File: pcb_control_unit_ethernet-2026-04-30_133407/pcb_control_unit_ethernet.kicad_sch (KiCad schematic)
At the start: 42 parts, among them J1 STDC14, J2 Micro_SD_Card_Det1, SW1 Reset, SW2 Boot, U1 STM32H563VITx, U10 SIT3051TK

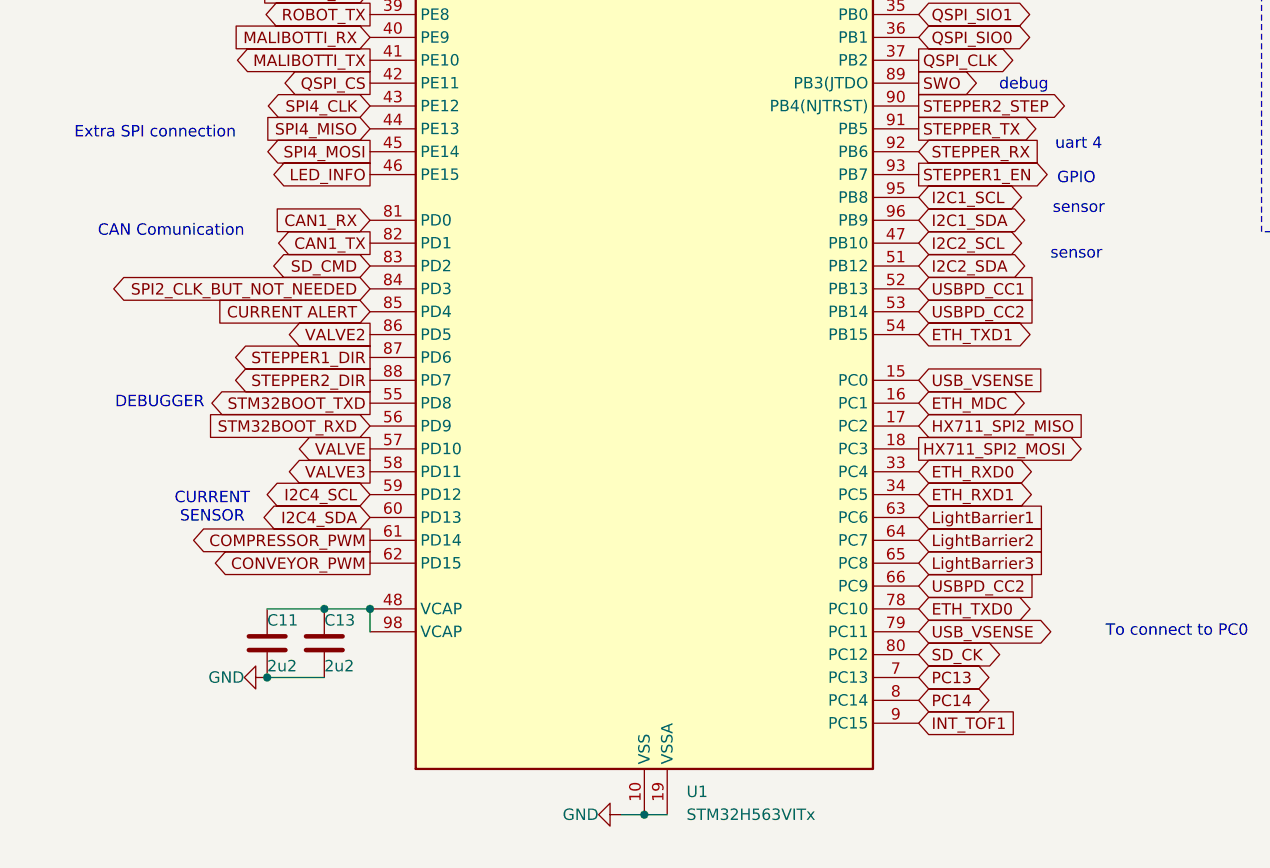
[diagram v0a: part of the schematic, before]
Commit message: WIP
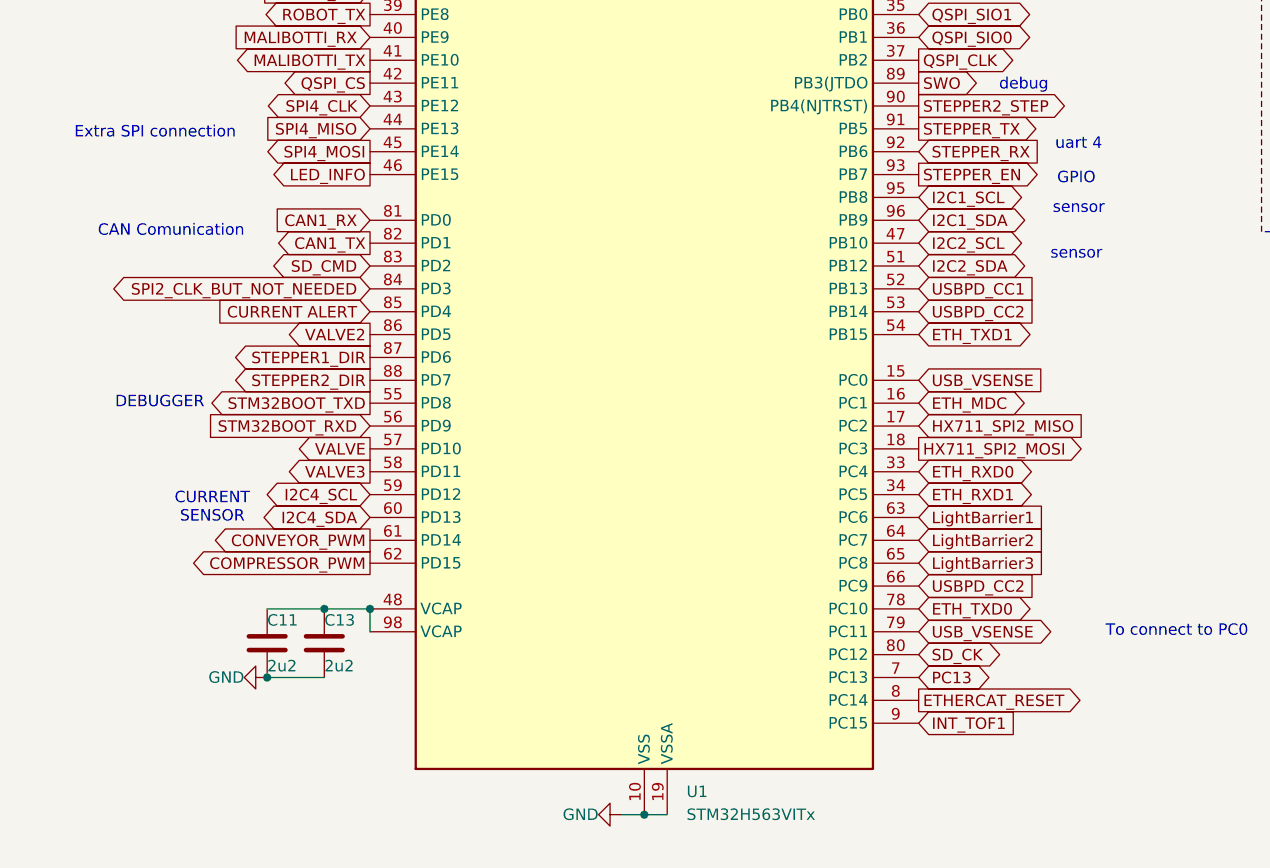
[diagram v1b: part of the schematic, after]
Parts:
- R1, R11, R12, R13, R14, R2, R3, R4, R5, R6, R63, R7, R8, R9: footprint Resistor_SMD:R_0201_0603Metric -> Resistor_SMD:R_0402_1005Metric
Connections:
- net COMPRESSOR_PWM: now also U1.62 (PD15); no longer U1.61 (PD14)
- net CONVEYOR_PWM: now also U1.61 (PD14); no longer U1.62 (PD15)
- net PC14 renamed ETHERCAT_RESET
- net STEPPER1_EN renamed STEPPER_EN

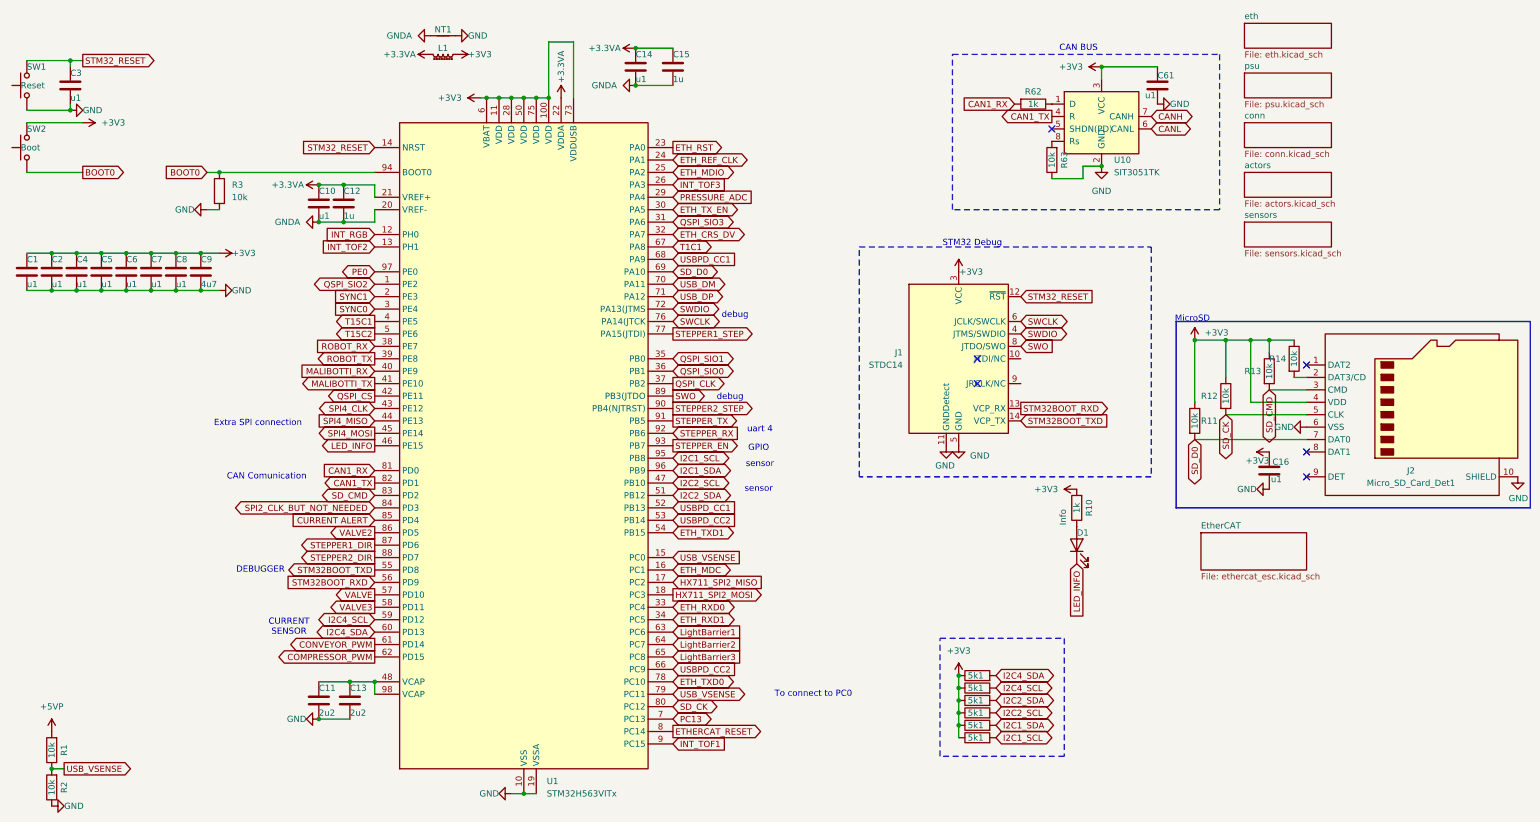
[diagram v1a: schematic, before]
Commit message: WIP
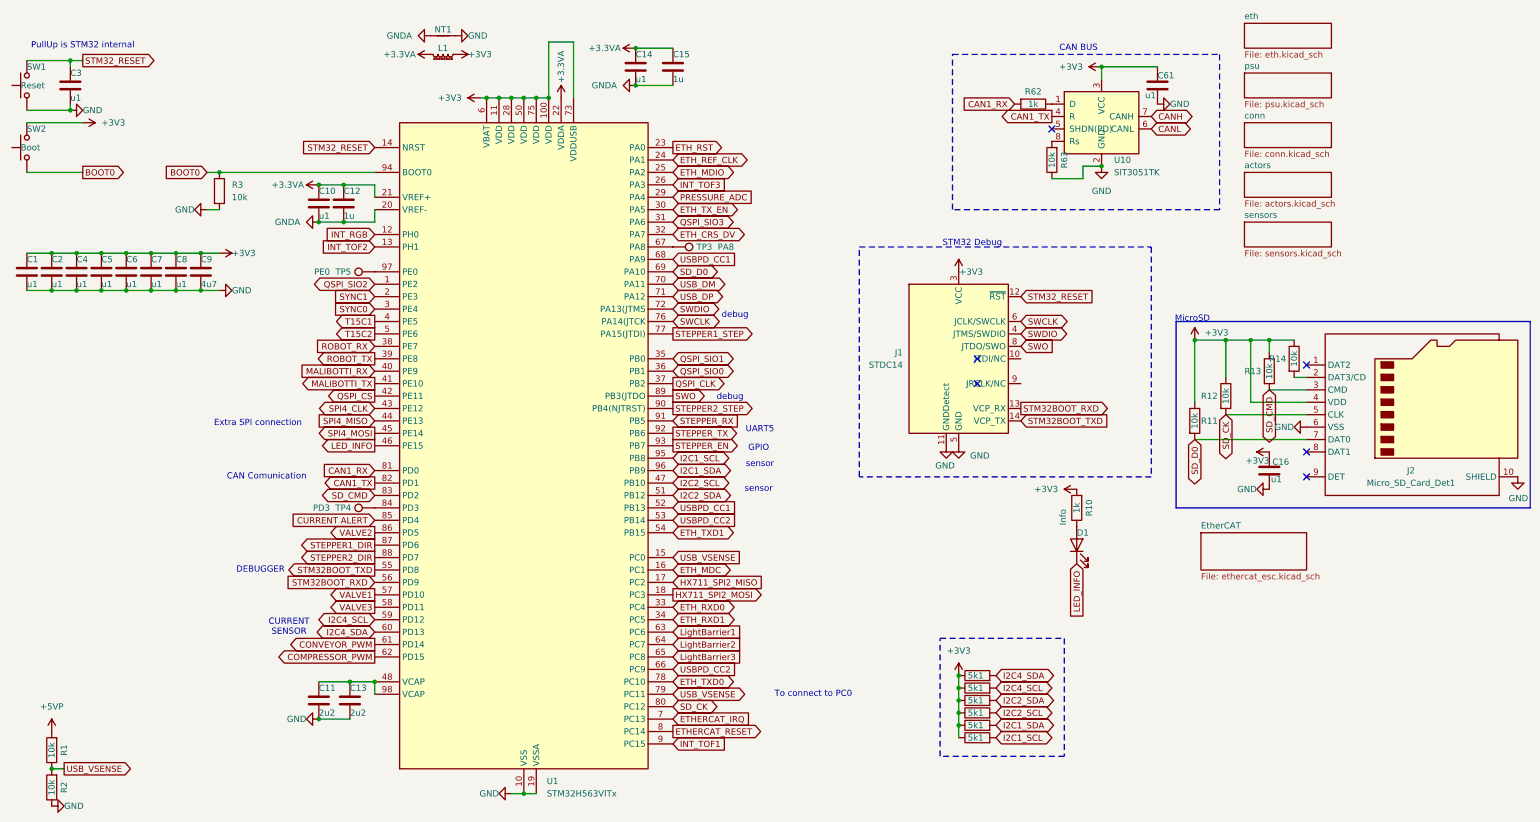
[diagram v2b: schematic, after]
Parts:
- added TP3: PA8, TestPoint:TestPoint_THTPad_D1.0mm_Drill0.5mm, symbol Connector:TestPoint
- added TP4: PD3, TestPoint:TestPoint_THTPad_D1.0mm_Drill0.5mm, symbol Connector:TestPoint
- added TP5: PE0, TestPoint:TestPoint_THTPad_D1.0mm_Drill0.5mm, symbol Connector:TestPoint
- L1: value 600R@100M -> 220R@100M
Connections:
- net STEPPER_RX: now also U1.91 (PB5); no longer U1.92 (PB6)
- net STEPPER_TX: now also U1.92 (PB6); no longer U1.91 (PB5)
- net PC13 renamed ETHERCAT_IRQ
- net PE0: no longer names the net of U1.97 (PE0)
- net PE0: now also TP5.1
- net SPI2_CLK_BUT_NOT_NEEDED: no longer names the net of U1.84 (PD3)
- net SPI2_CLK_BUT_NOT_NEEDED: now also TP4.1
- net T1C1: no longer names the net of U1.67 (PA8)
- net T1C1: now also TP3.1
- net VALVE renamed VALVE1
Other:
- note added: "PullUp is STM32 internal"
- note added: "UART5"
- note removed: "uart 4"
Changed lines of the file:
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@@
 (kicad_sch
-	(version 20250114)
+	(version 20260306)
 	(generator "eeschema")
-	(generator_version "9.0")
+	(generator_version "10.0")
 	(paper "A4")

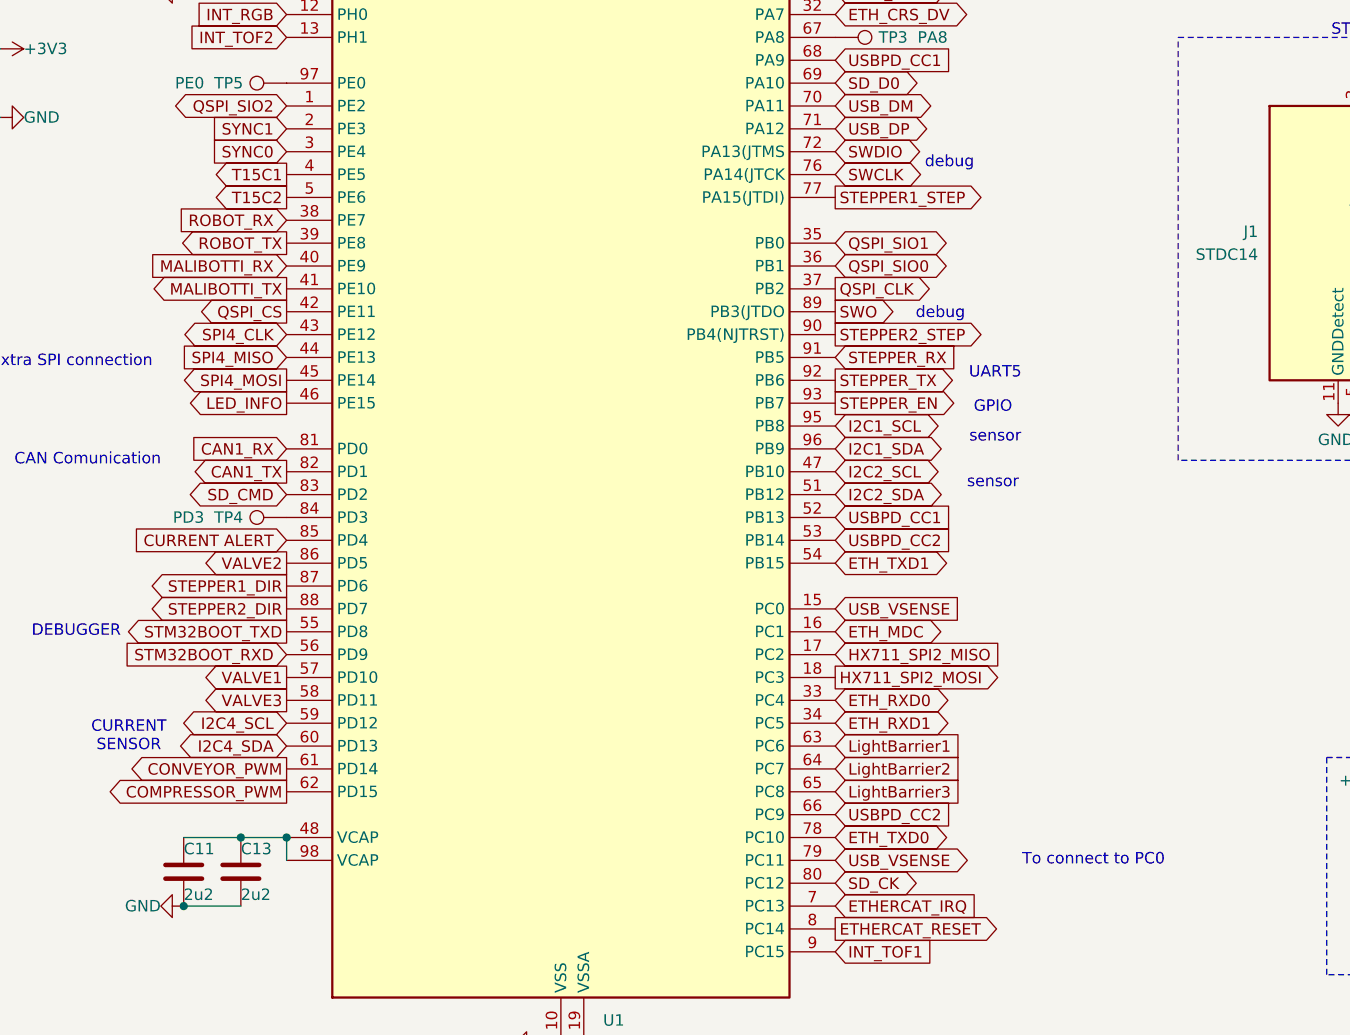
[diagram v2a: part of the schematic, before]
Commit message: Release Candidate
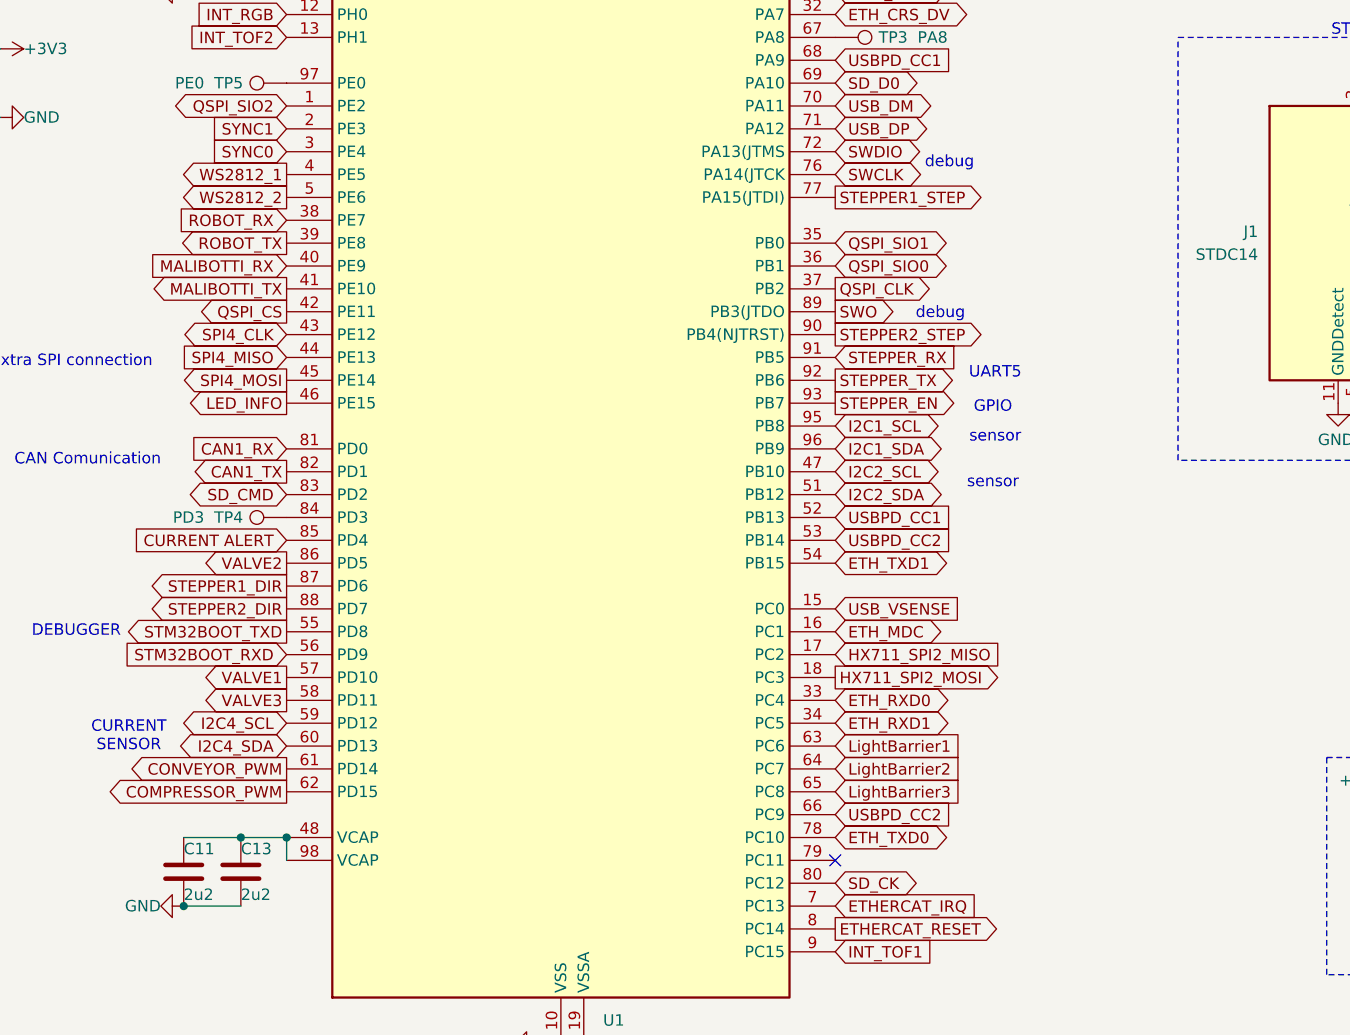
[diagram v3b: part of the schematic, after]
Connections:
- net USB_VSENSE: no longer U1.79 (PC11)
- net T15C1 renamed WS2812_1
- net T15C2 renamed WS2812_2
- no-connect marks 6 -> 7
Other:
- note removed: "To connect to PC0"
